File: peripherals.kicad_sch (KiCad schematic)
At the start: 73 parts, among them J10 AudioJack3, J11 AudioJack3, J13 Joy, J14 Video Out, J15 DB15_Female_HighDensity, J3 Mini-DIN-6, J4 Mini-DIN-6, Q1 BC846, Q2 BC846, U2 PCM5102

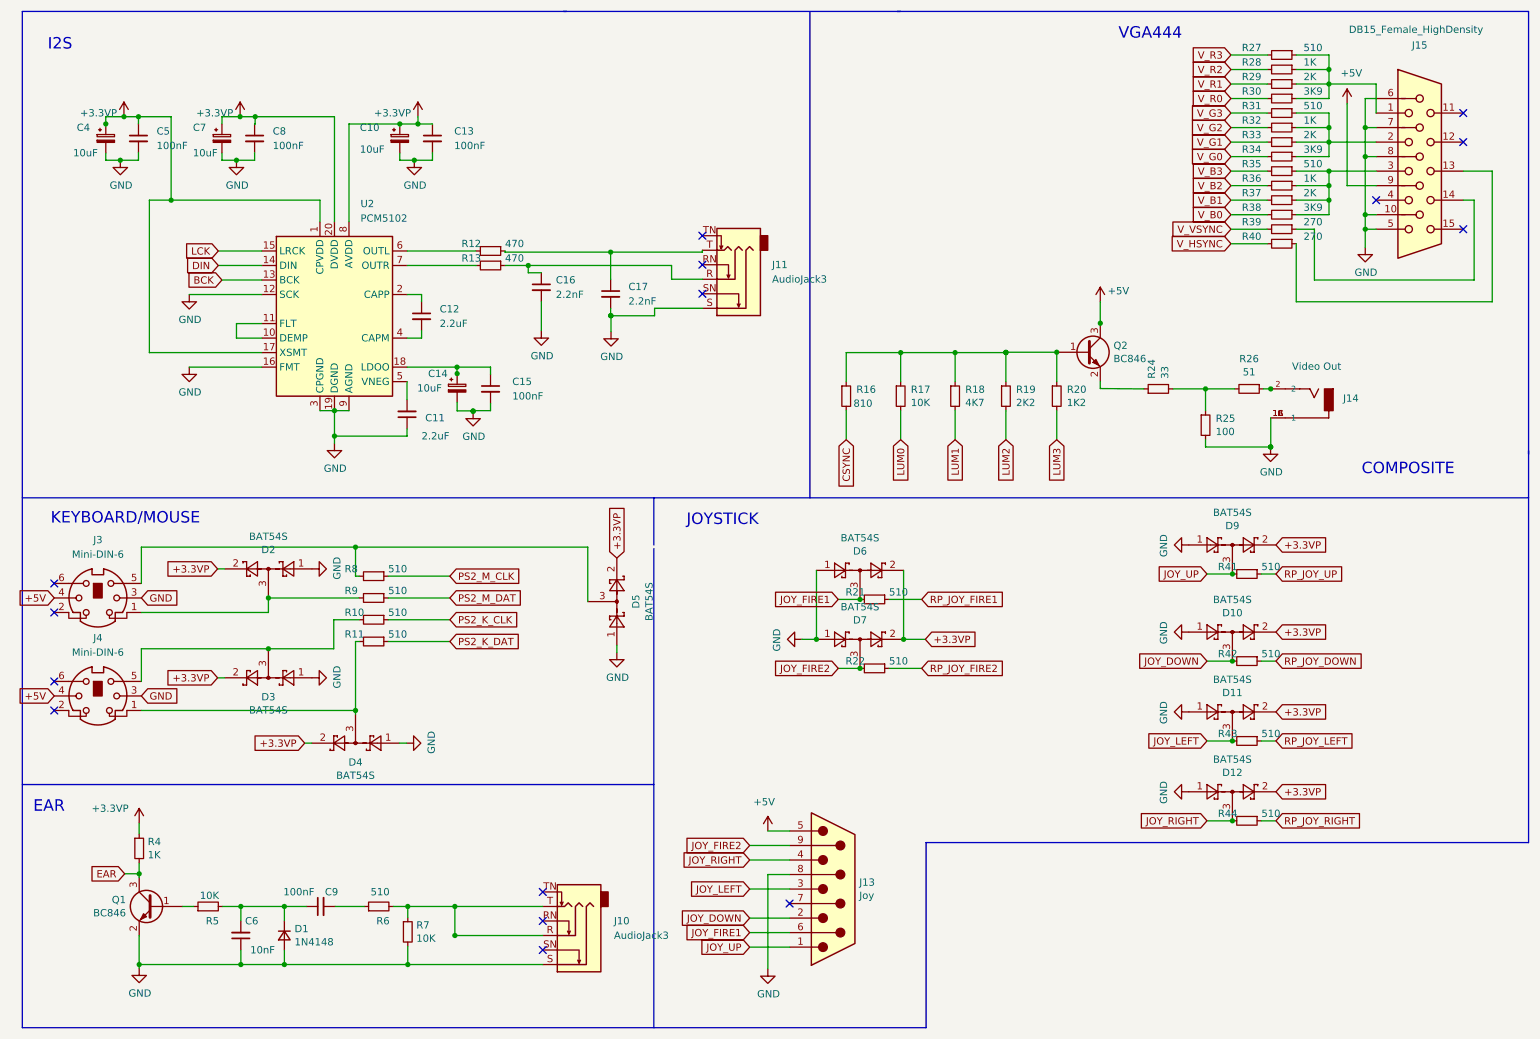
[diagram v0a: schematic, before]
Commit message: test
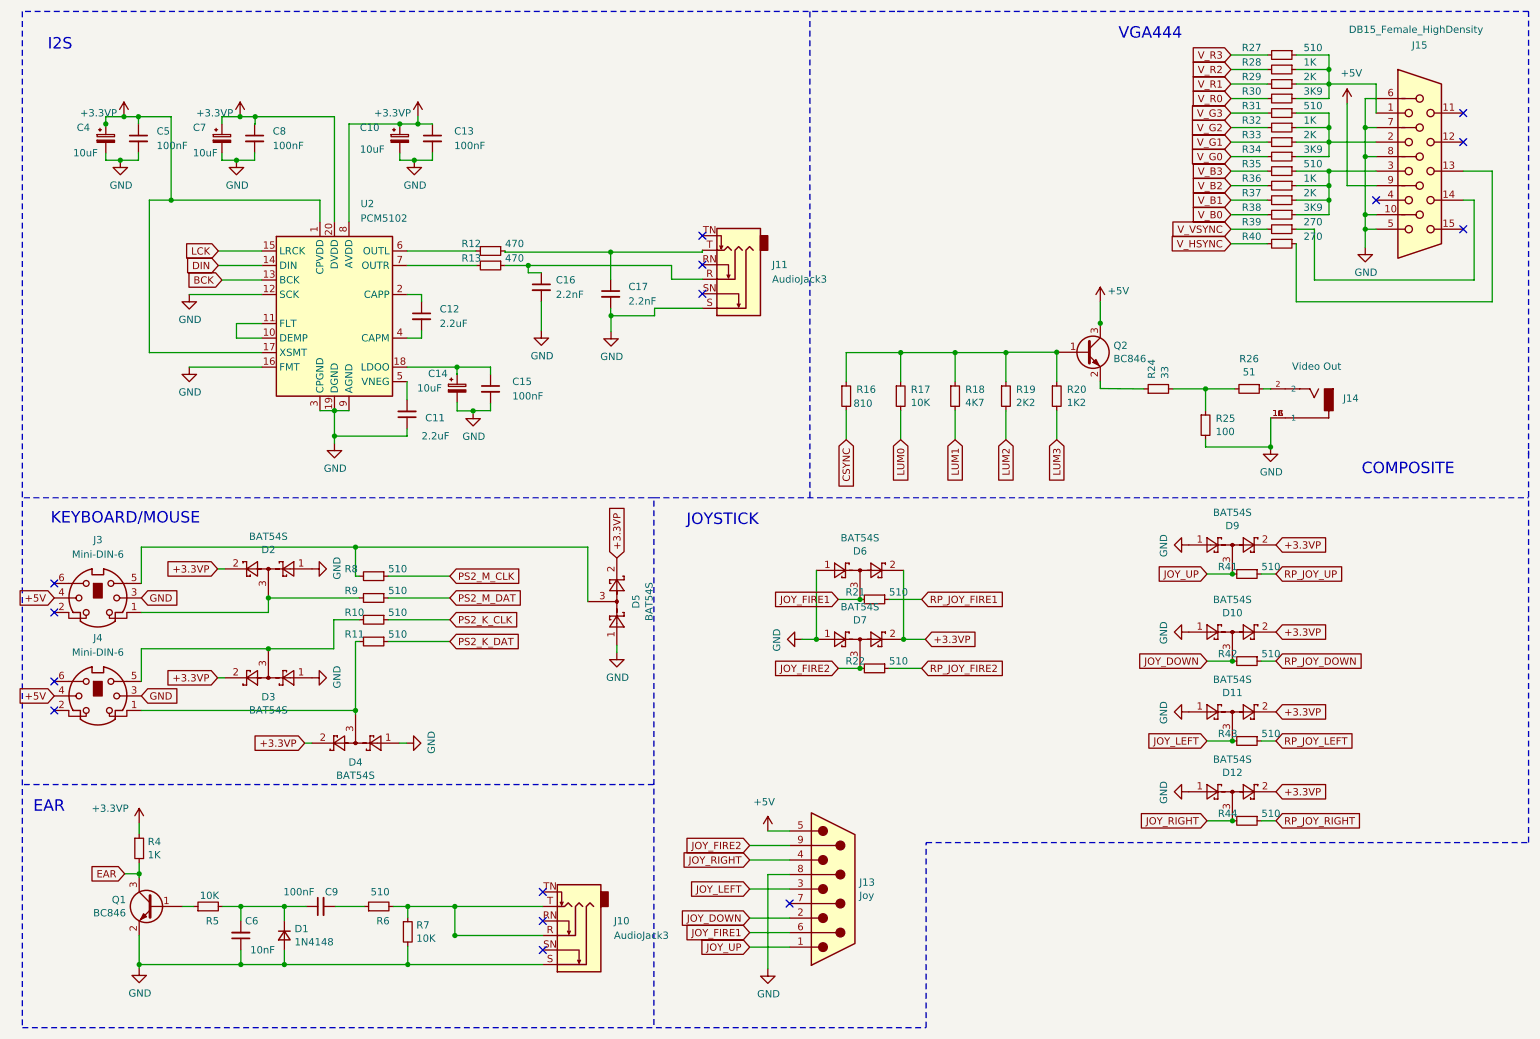
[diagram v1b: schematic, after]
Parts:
- C10, C14, C4: LCSC (none) -> C7171
- C11, C12: footprint Capacitor_SMD:C_1206_3216Metric_Pad1.33x1.80mm_HandSolder -> Capacitor_SMD:C_0805_2012Metric_Pad1.18x1.45mm_HandSolder; LCSC (none) -> C377773
- C13, C15, C5, C8, C9: footprint Capacitor_SMD:C_1206_3216Metric_Pad1.33x1.80mm_HandSolder -> Capacitor_SMD:C_0805_2012Metric_Pad1.18x1.45mm_HandSolder; LCSC (none) -> C28233
- C16, C17: footprint Capacitor_SMD:C_1206_3216Metric_Pad1.33x1.80mm_HandSolder -> Capacitor_SMD:C_0805_2012Metric_Pad1.18x1.45mm_HandSolder; LCSC (none) -> C36576
- C6: footprint Capacitor_SMD:C_1206_3216Metric_Pad1.33x1.80mm_HandSolder -> Capacitor_SMD:C_0805_2012Metric_Pad1.18x1.45mm_HandSolder; LCSC (none) -> C1710
- C7: footprint Capacitor_SMD:C_1206_3216Metric_Pad1.33x1.80mm_HandSolder -> Capacitor_Tantalum_SMD:CP_EIA-3216-12_Kemet-S_Pad1.58x1.35mm_HandSolder; LCSC (none) -> C7171
- D1: footprint Diode_SMD:D_MiniMELF -> Diode_SMD:D_SOD-123F; LCSC (none) -> C81598
- D10, D11, D12, D2, D3, D4, D5, D6, D7, D9: LCSC (none) -> C181201
- Q1, Q2: LCSC (none) -> C779722
- R10, R11, R21, R22, R27, R31, R35, R41, R42, R43, R44, R6, R8, R9: footprint Resistor_SMD:R_1206_3216Metric_Pad1.30x1.75mm_HandSolder -> Resistor_SMD:R_0805_2012Metric_Pad1.20x1.40mm_HandSolder; LCSC (none) -> C17734
- R12, R13: footprint Resistor_SMD:R_1206_3216Metric_Pad1.30x1.75mm_HandSolder -> Resistor_SMD:R_0805_2012Metric_Pad1.20x1.40mm_HandSolder; LCSC (none) -> C17710
- R16: footprint Resistor_SMD:R_1206_3216Metric_Pad1.30x1.75mm_HandSolder -> Resistor_SMD:R_0805_2012Metric_Pad1.20x1.40mm_HandSolder
- R17, R5, R7: footprint Resistor_SMD:R_1206_3216Metric_Pad1.30x1.75mm_HandSolder -> Resistor_SMD:R_0805_2012Metric_Pad1.20x1.40mm_HandSolder; LCSC (none) -> C17414
- R18: footprint Resistor_SMD:R_1206_3216Metric_Pad1.30x1.75mm_HandSolder -> Resistor_SMD:R_0805_2012Metric_Pad1.20x1.40mm_HandSolder; LCSC (none) -> C26022
- R19: footprint Resistor_SMD:R_1206_3216Metric_Pad1.30x1.75mm_HandSolder -> Resistor_SMD:R_0805_2012Metric_Pad1.20x1.40mm_HandSolder; LCSC (none) -> C2907303
- R20: footprint Resistor_SMD:R_1206_3216Metric_Pad1.30x1.75mm_HandSolder -> Resistor_SMD:R_0805_2012Metric_Pad1.20x1.40mm_HandSolder; LCSC (none) -> C17379
- R24: footprint Resistor_SMD:R_1206_3216Metric_Pad1.30x1.75mm_HandSolder -> Resistor_SMD:R_0805_2012Metric_Pad1.20x1.40mm_HandSolder; LCSC (none) -> C17634
- R25: footprint Resistor_SMD:R_1206_3216Metric_Pad1.30x1.75mm_HandSolder -> Resistor_SMD:R_0805_2012Metric_Pad1.20x1.40mm_HandSolder; LCSC (none) -> C115423
- R26: footprint Resistor_SMD:R_1206_3216Metric_Pad1.30x1.75mm_HandSolder -> Resistor_SMD:R_0805_2012Metric_Pad1.20x1.40mm_HandSolder; LCSC (none) -> C17738
- R28, R32, R36, R4: footprint Resistor_SMD:R_1206_3216Metric_Pad1.30x1.75mm_HandSolder -> Resistor_SMD:R_0805_2012Metric_Pad1.20x1.40mm_HandSolder; LCSC (none) -> C17513
- R29, R33, R37: footprint Resistor_SMD:R_1206_3216Metric_Pad1.30x1.75mm_HandSolder -> Resistor_SMD:R_0805_2012Metric_Pad1.20x1.40mm_HandSolder; LCSC (none) -> C2907315
- R30, R34, R38: footprint Resistor_SMD:R_1206_3216Metric_Pad1.30x1.75mm_HandSolder -> Resistor_SMD:R_0805_2012Metric_Pad1.20x1.40mm_HandSolder; LCSC (none) -> C17614
- R39, R40: footprint Resistor_SMD:R_1206_3216Metric_Pad1.30x1.75mm_HandSolder -> Resistor_SMD:R_0805_2012Metric_Pad1.20x1.40mm_HandSolder; LCSC (none) -> C2907313
- U2: LCSC (none) -> C1520792
